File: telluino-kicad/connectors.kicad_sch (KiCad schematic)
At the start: 11 parts, among them U3 DS2433S+

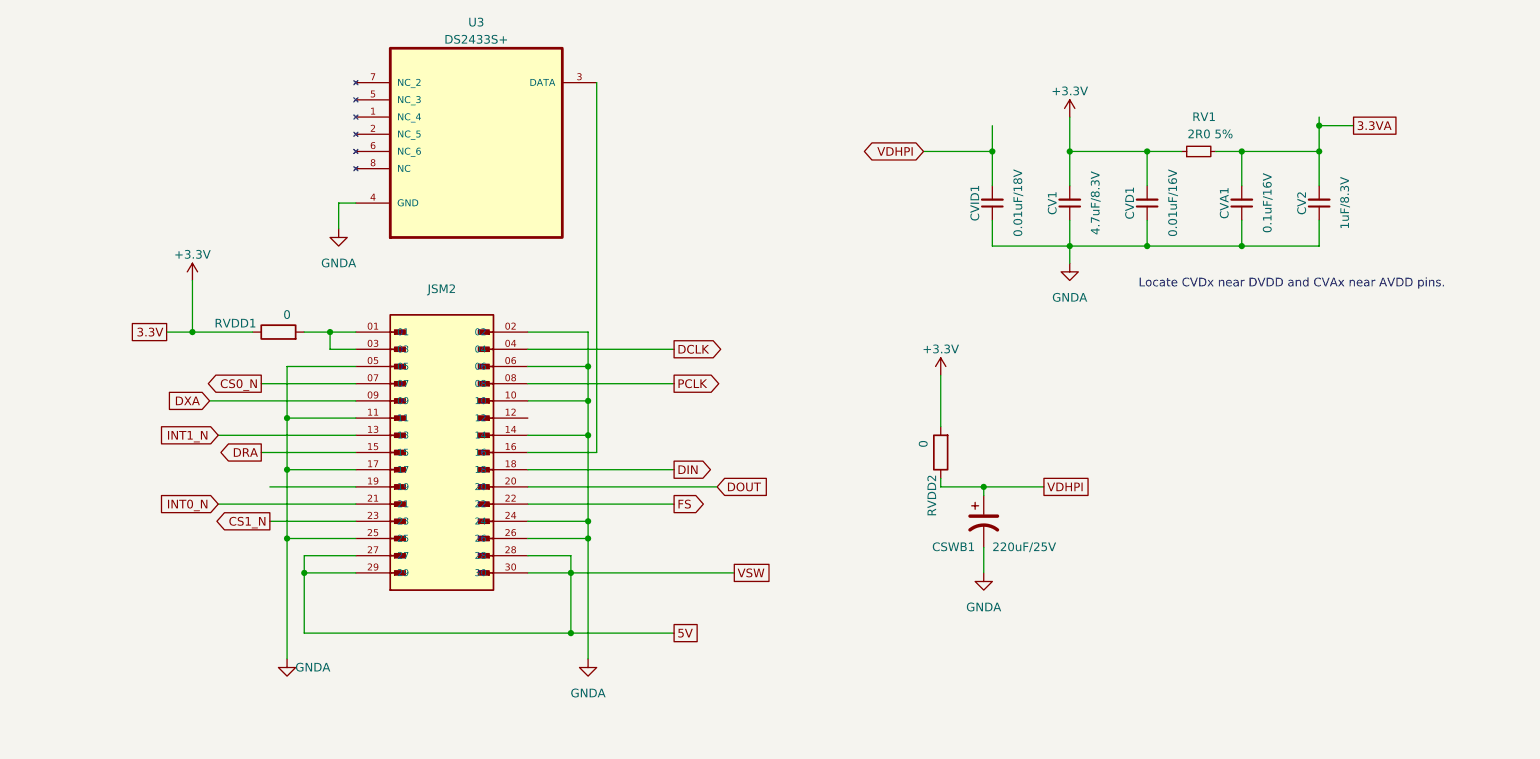
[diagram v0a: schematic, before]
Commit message: schematic done
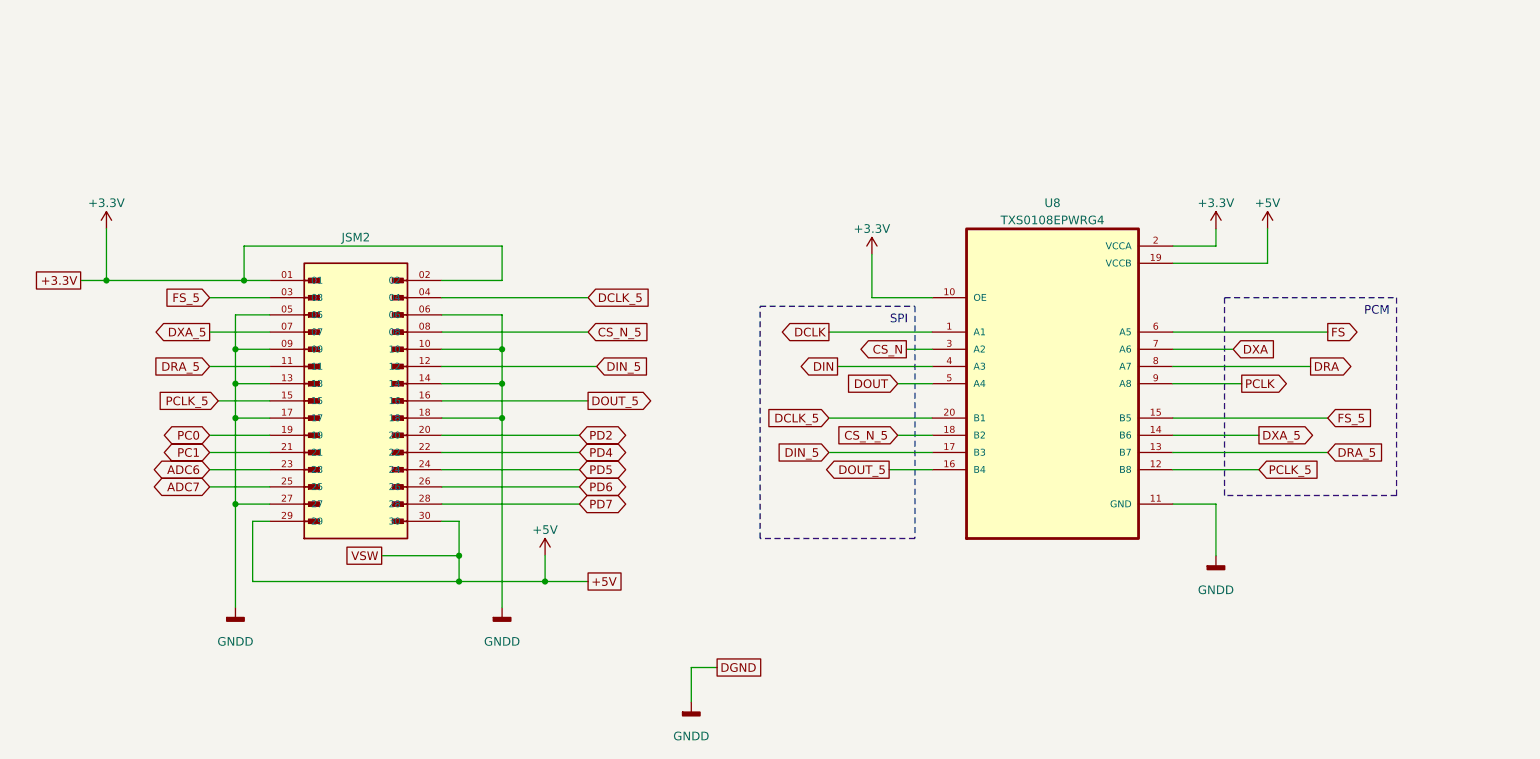
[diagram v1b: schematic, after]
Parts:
- removed CSWB1: 220uF/25V, Capacitor_THT:CP_Radial_D10.0mm_P2.50mm, symbol Device:C_Polarized_US
- removed CV1: 4.7uF/8.3V, Capacitor_SMD:C_0201_0603Metric_Pad0.64x0.40mm_HandSolder, symbol Device:C_Small
- removed CV2: 1uF/8.3V, Capacitor_SMD:C_0201_0603Metric_Pad0.64x0.40mm_HandSolder, symbol Device:C_Small
- removed CVA1: 0.1uF/16V, Capacitor_SMD:C_0201_0603Metric_Pad0.64x0.40mm_HandSolder, symbol Device:C_Small
- removed CVD1: 0.01uF/16V, Capacitor_SMD:C_0201_0603Metric_Pad0.64x0.40mm_HandSolder, symbol Device:C_Small
- removed CVID1: 0.01uF/18V, Capacitor_SMD:C_0201_0603Metric_Pad0.64x0.40mm_HandSolder, symbol Device:C_Small
- removed RV1: 2R0 5%, Resistor_THT:R_Axial_DIN0309_L9.0mm_D3.2mm_P12.70mm_Horizontal, symbol Device:R_Small
- removed RVDD1, RVDD2: 0, Resistor_SMD:R_0603_1608Metric_Pad0.98x0.95mm_HandSolder, symbol Device:R
- removed U3: DS2433S+, my_lib:SOIC127P780X210-8N, symbol my_lib:DS2433S+
- added U8: TXS0108EPWRG4, my_lib:SOP65P640X120-20N, symbol TXS0108:TXS0108EPWRG4
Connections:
- net INT1_N is gone; now on net GNDD: JSM2.13
- net +3.3V: now also JSM2.01, JSM2.02, U8.10 (OE), U8.2 (VCCA)
- net DCLK: now also U8.1 (A1); no longer JSM2.04
- net DIN: now also U8.4 (A3); no longer JSM2.18
- net DOUT: now also U8.5 (A4); no longer JSM2.20
- net DRA: now also U8.8 (A7); no longer JSM2.15
- net DXA: now also U8.7 (A6); no longer JSM2.09
- net FS: now also U8.6 (A5); no longer JSM2.22
- net PCLK: now also U8.9 (A8); no longer JSM2.08
- net FS_5: now reaches JSM2.03
- net FS_5: now also U8.15 (B5); no longer JSM2.01
- net DIN_5: now reaches JSM2.12
- net DIN_5: now also U8.17 (B3)
- net DOUT_5: now reaches JSM2.16
- net DOUT_5: now also U8.16 (B4)
- net PC0: now reaches JSM2.19
- net 5V renamed +5V
- net +5V: now also U8.19 (VCCB); no longer JSM2.27, JSM2.28
- net CS0_N renamed DXA_5
- net DXA_5: now also U8.14 (B6)
- net CS1_N renamed ADC6
- net GNDA renamed GNDD
- net GNDD: now also JSM2.09, JSM2.18, JSM2.27, U8.11 (GND); no longer JSM2.02, JSM2.11, JSM2.24, JSM2.25, JSM2.26
- net INT0_N renamed PC1
- new net ADC7: JSM2.25
- new net CS_N: U8.3 (A2)
- new net CS_N_5: JSM2.08, U8.18 (B2)
- new net DCLK_5: JSM2.04, U8.20 (B1)
- new net DRA_5: JSM2.11, U8.13 (B7)
- new net PCLK_5: JSM2.15, U8.12 (B8)
- new net PD2: JSM2.20
- new net PD4: JSM2.22
- new net PD5: JSM2.24
- new net PD6: JSM2.26
- new net PD7: JSM2.28
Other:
- note removed: "Locate CVDx near DVDD and CVAx near AVDD pins."
- moved on the sheet: JSM2

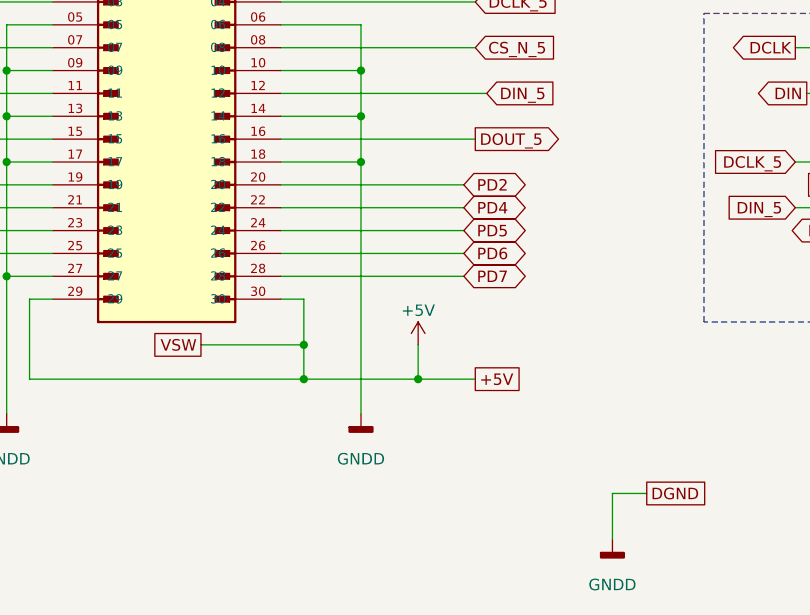
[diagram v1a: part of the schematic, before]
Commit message: ready_placement
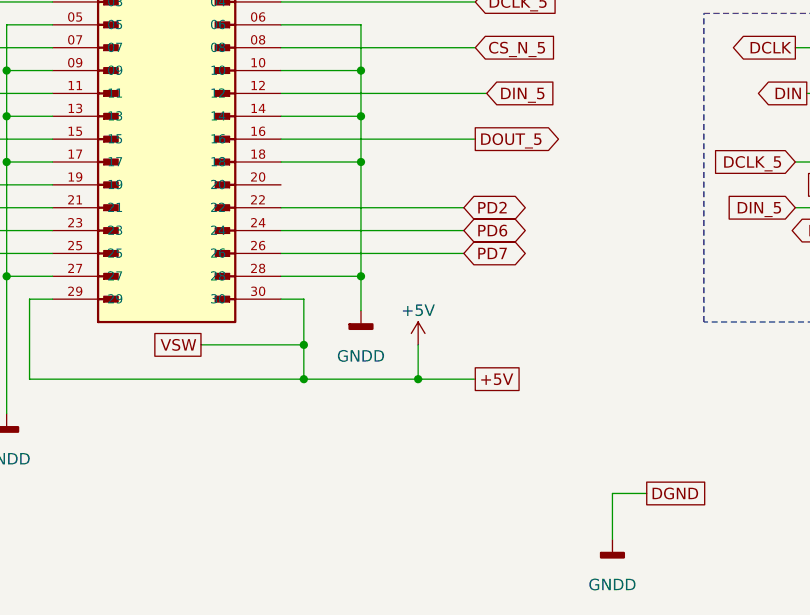
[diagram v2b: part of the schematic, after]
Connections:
- net PD4 is gone; now on net PD2: JSM2.22
- net PD5 is gone; now on net PD6: JSM2.24
- net GNDD: now also JSM2.28
- net PD2: no longer JSM2.20
- net PD6: no longer JSM2.26
- net PD7: now also JSM2.26; no longer JSM2.28
